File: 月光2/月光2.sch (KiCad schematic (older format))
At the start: 73 parts, among them J1 Conn_01x12, J2 Conn_01x12, J3 Conn_01x05, J4 Conn_01x03, J6 Conn_01x02, Q1 Q_Photo_NPN, Q2 Q_Photo_NPN, Q3 Q_Photo_NPN, Q4 Q_Photo_NPN, Q5 IRLML6344TRPBFTR, SW1 SW_Push_Dual_x2, U1 DRV8835, U2 STM32F413CH6, U4 LP5907_DBV, U5 ICM20648, Y1 Crystal_GND23

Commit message: #
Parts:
- D1, D3, Q2, Q3: footprint LED_THT:LED_D3.0mm_Horizontal_O3.81mm_Z2.0mm -> micro:micro_reverce_LED
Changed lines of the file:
@@
 F 0 "D1" V 3538 7133 50  0000 R CNN
 F 1 "LED" V 3447 7133 50  0000 R CNN
-F 2 "LED_THT:LED_D3.0mm_Horizontal_O3.81mm_Z2.0mm" H 3500 7250 50  0001 C CNN
+F 2 "micro:micro_reverce_LED" H 3500 7250 50  0001 C CNN
 F 3 "~" H 3500 7250 50  0001 C CNN
 	1    3500 7250
@@
 F 0 "D3" V 4138 7133 50  0000 R CNN
 F 1 "LED" V 4047 7133 50  0000 R CNN
-F 2 "LED_THT:LED_D3.0mm_Horizontal_O3.81mm_Z2.0mm" H 4100 7250 50  0001 C CNN
+F 2 "micro:micro_reverce_LED" H 4100 7250 50  0001 C CNN
 F 3 "~" H 4100 7250 50  0001 C CNN
 	1    4100 7250
@@
 F 0 "Q2" H 1390 6446 50  0000 L CNN
 F 1 "Q_Photo_NPN" V 1150 5750 50  0000 L CNN
-F 2 "LED_THT:LED_D3.0mm_Horizontal_O3.81mm_Z2.0mm" H 1400 6500 50  0001 C CNN
+F 2 "micro:micro_reverce_LED" H 1400 6500 50  0001 C CNN
 F 3 "~" H 1200 6400 50  0001 C CNN
 	1    1200 6400
@@
 F 0 "Q3" H 1890 6446 50  0000 L CNN
 F 1 "Q_Photo_NPN" V 1650 5750 50  0000 L CNN
-F 2 "LED_THT:LED_D3.0mm_Horizontal_O3.81mm_Z2.0mm" H 1900 6500 50  0001 C CNN
+F 2 "micro:micro_reverce_LED" H 1900 6500 50  0001 C CNN
 F 3 "~" H 1700 6400 50  0001 C CNN
 	1    1700 6400

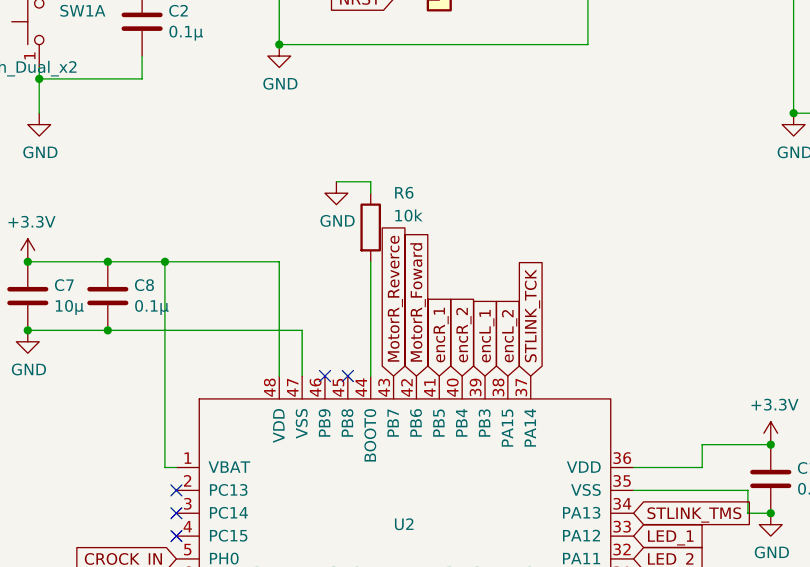
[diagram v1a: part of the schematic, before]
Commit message: finish
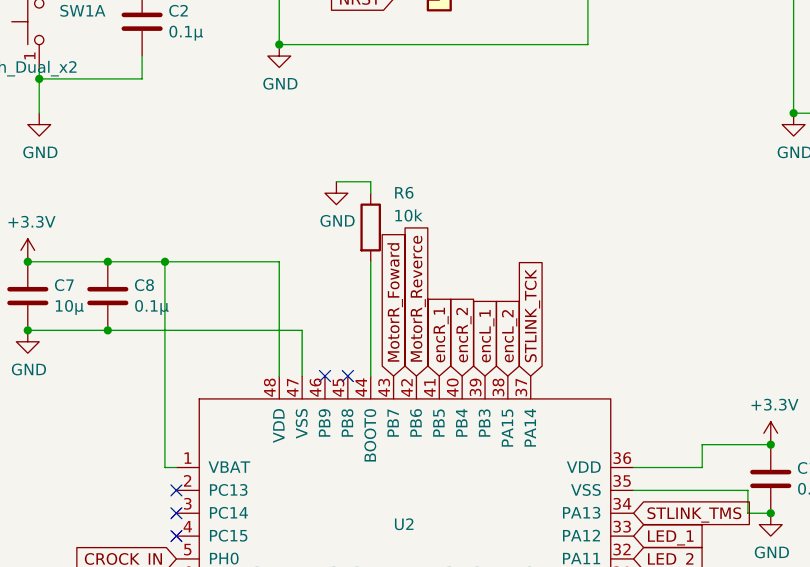
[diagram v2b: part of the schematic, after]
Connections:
- net MotorR_Foward: now also U2.43 (PB7); no longer U2.42 (PB6)
- net MotorR_Reverce: now also U2.42 (PB6); no longer U2.43 (PB7)
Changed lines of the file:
@@
 Wire Wire Line
 	2250 1900 2400 1900
+Text GLabel 6100 3200 1    50   Input ~ 0
+MotorR_Reverce
 Text GLabel 6000 3200 1    50   Input ~ 0
-MotorR_Reverce
-Text GLabel 6100 3200 1    50   Input ~ 0
 MotorR_Foward
 Text GLabel 5050 4500 0    50   Input ~ 0
